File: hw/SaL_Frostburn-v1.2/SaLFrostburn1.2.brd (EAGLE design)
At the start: 72.7 x 19.8 mm, 99 parts, among them U1 ATSAMD21G-A, U3 ADXL345, U4 gps, Y1 32.768kHx, Y3 32MHz

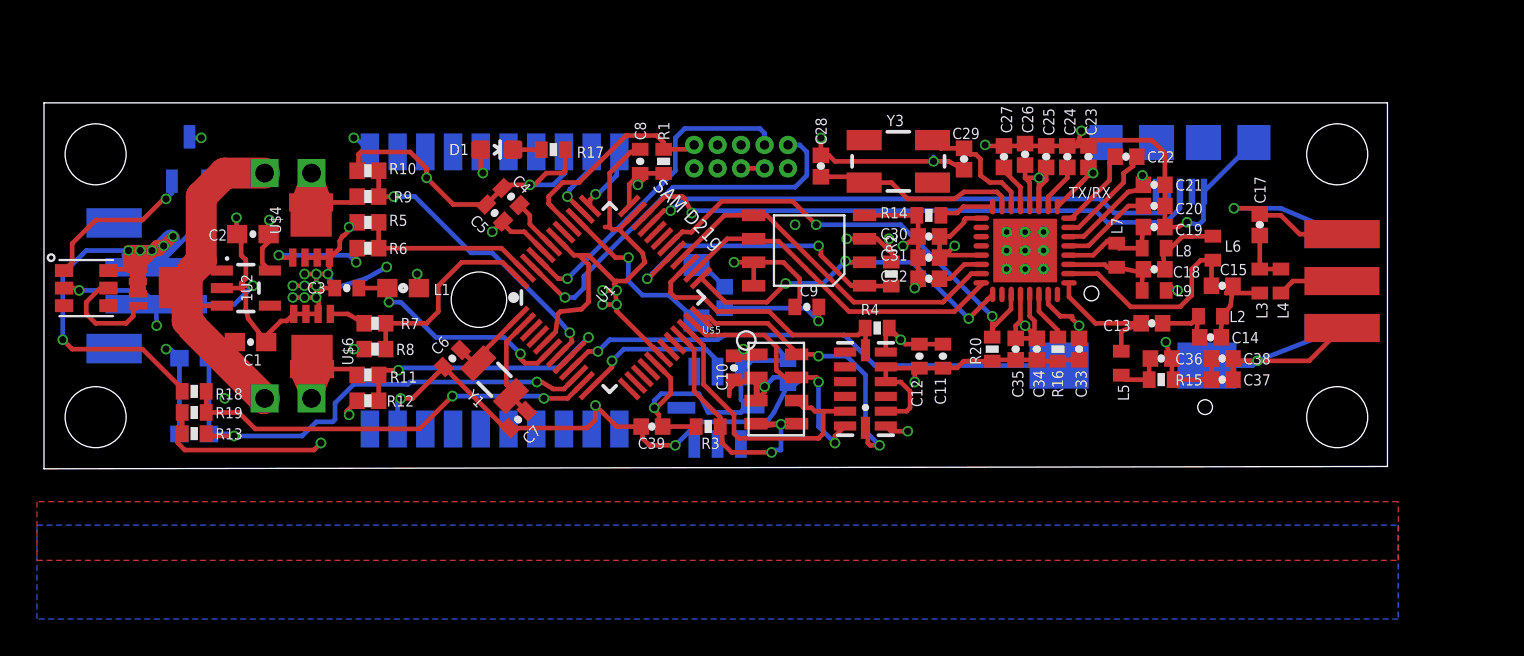
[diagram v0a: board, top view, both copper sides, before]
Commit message: 1.2 hw sent to fab and some work on 1.1 code
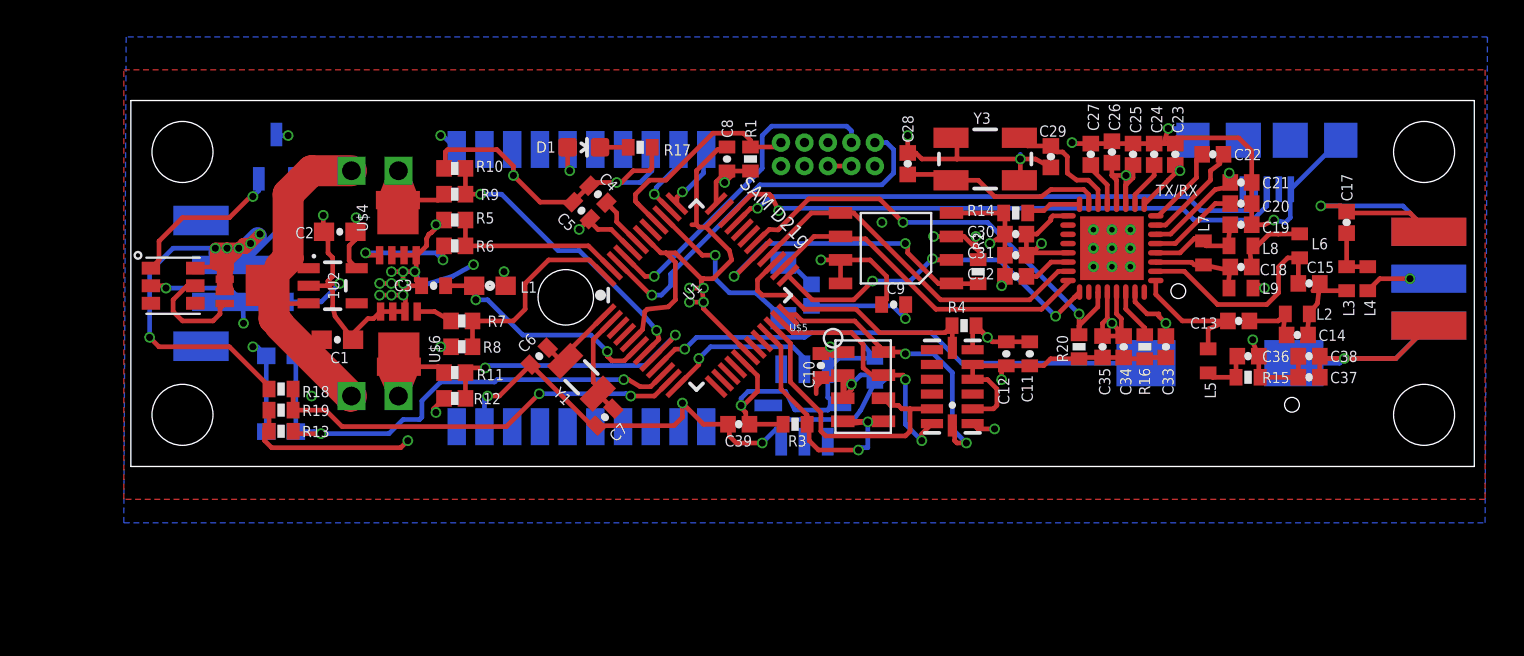
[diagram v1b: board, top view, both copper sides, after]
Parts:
- removed FRAME1: FRAME-LEDGER, SparkFun-Aesthetics:CREATIVE_COMMONS
- moved C12 4.70 mm to (47.4, 6.10)
- moved C13 4.70 mm to (59.9, 7.87)
- moved C35 4.70 mm to (52.6, 6.48)
- moved JP4 4.70 mm to (61.5, 17.7)
- moved L4 4.70 mm to (66.9, 10.2)
- moved L6 4.70 mm to (63.2, 11.9)
- moved U$5 4.70 mm to (39.6, 4.32)
- moved U3 4.70 mm to (44.5, 4.32)
- moved C39 4.70 mm to (32.9, 2.29)
- moved C5 4.70 mm to (24.4, 13.8)
- moved C7 4.70 mm to (25.7, 2.67)
- moved C8 4.70 mm to (32.3, 16.6)
- moved L1 4.70 mm to (19.4, 9.78)
- moved R17 4.70 mm to (27.6, 17.3)
- moved R3 4.70 mm to (35.9, 2.29)
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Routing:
- net GND: track 358.6 -> 362.1 mm
- net N$13: vias 0 -> 1
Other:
- outline, holes or cut-outs redrawn
- board text added: "SaLFrostburn V1.2"
- board text removed: "SaLFrostburn V1.1"
